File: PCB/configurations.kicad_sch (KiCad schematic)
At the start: 18 parts, among them J2 Conn_ARM_SWD_TagConnect_TC2030, J3 USB_C_Receptacle_USB2.0_16P, U1 XC7A50T-FGG484, U3 FT2232HQ, Y1 12M

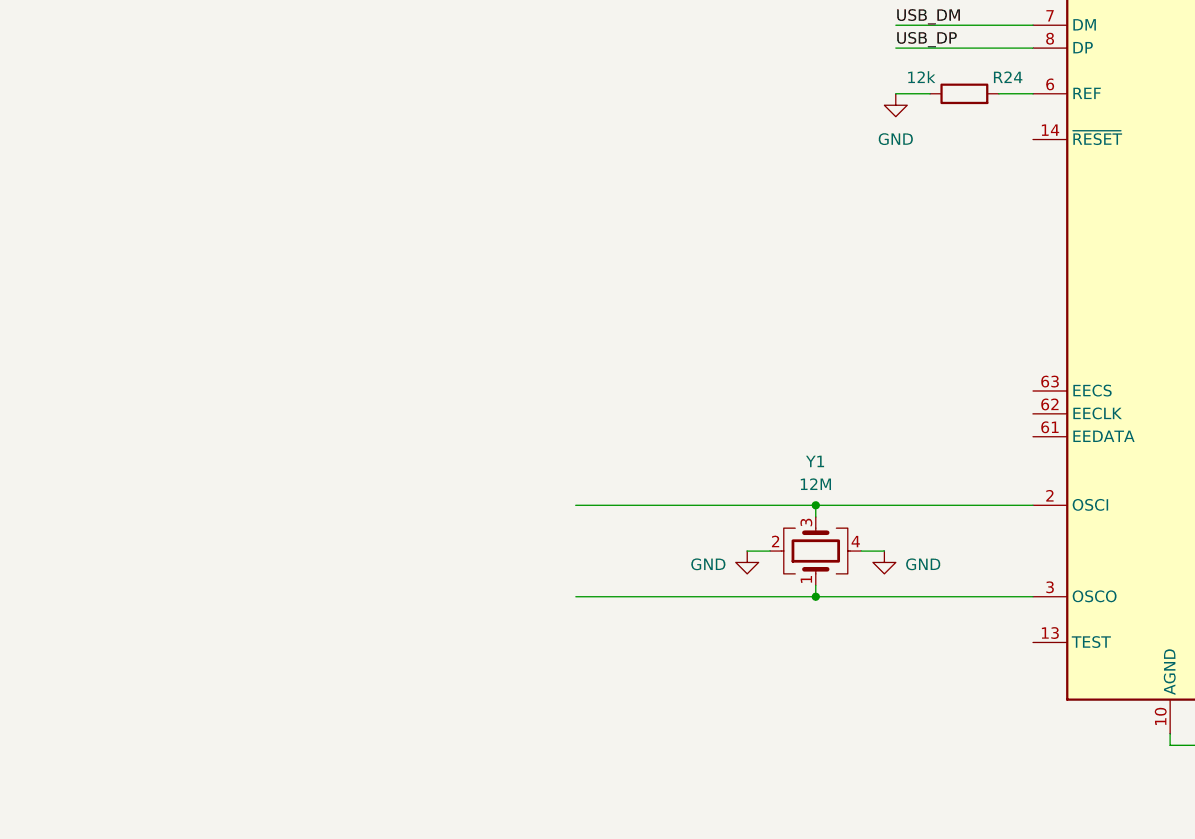
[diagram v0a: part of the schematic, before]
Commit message: adding EEPROM to FT2232H, more FT wiring too
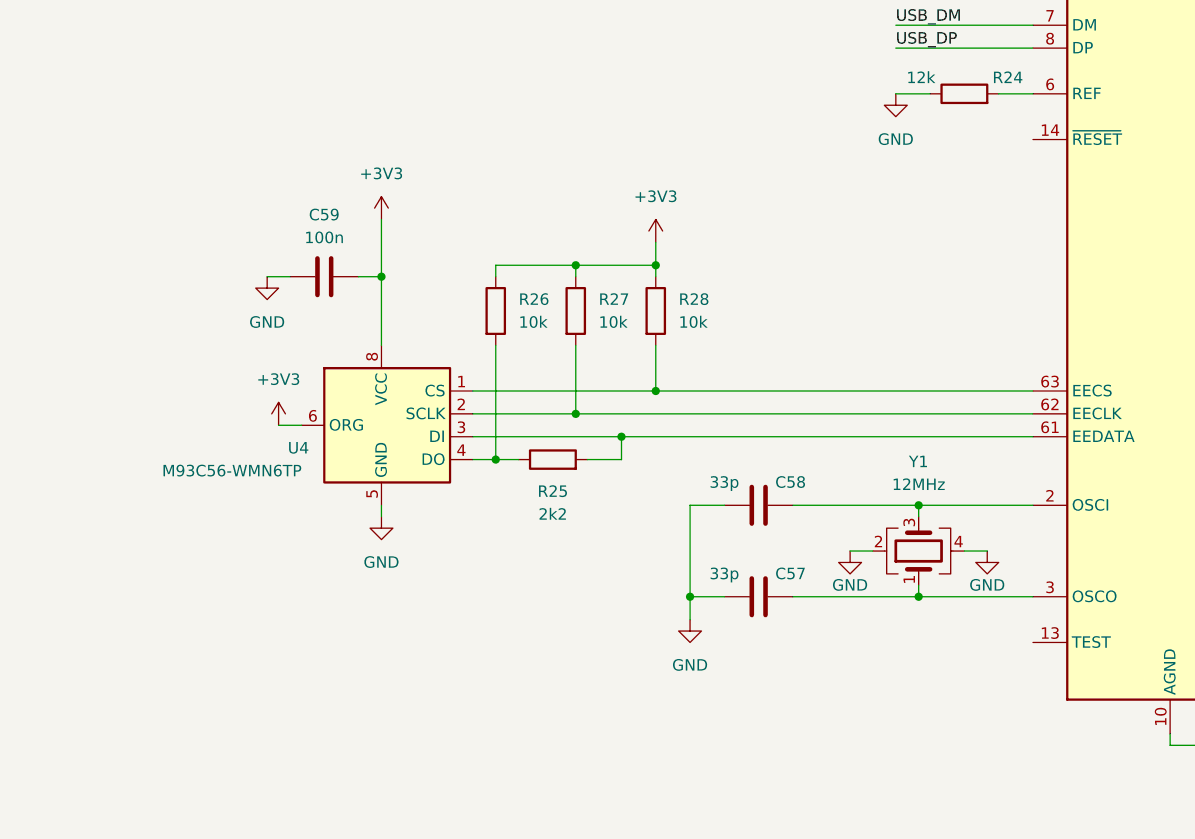
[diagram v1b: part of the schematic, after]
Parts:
- added C57, C58: 33p, symbol Device:C
- added C59: 100n, symbol Device:C
- added R25: 2k2, symbol Device:R
- added R26, R27, R28: 10k, symbol Device:R
- added U4: M93C56-WMN6TP, Package_SO:SOIC-8_3.9x4.9mm_P1.27mm, symbol FPGA Accelerator:M93C56-WMN6TP
- Y1: value 12M -> 12MHz
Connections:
- net +3V3: now also C59.2, R26.1, R27.1, R28.1, U4.6 (ORG), U4.8 (VCC)
- net GND: now also C57.1, C58.1, C59.1, U4.5 (GND)
- net at U3.3 (OSCO), Y1.1: now also C57.2
- net at U3.2 (OSCI), Y1.3: now also C58.2
- net at U3.61 (EEDATA): now also R25.2, U4.3 (DI)
- net at U3.62 (EECLK): now also R27.2, U4.2 (SCLK)
- net at U3.63 (EECS): now also R28.2, U4.1 (CS)
- new net: R25.1, R26.2, U4.4 (DO)
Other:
- moved on the sheet: Y1
